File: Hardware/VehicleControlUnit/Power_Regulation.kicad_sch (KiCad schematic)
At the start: 3 parts

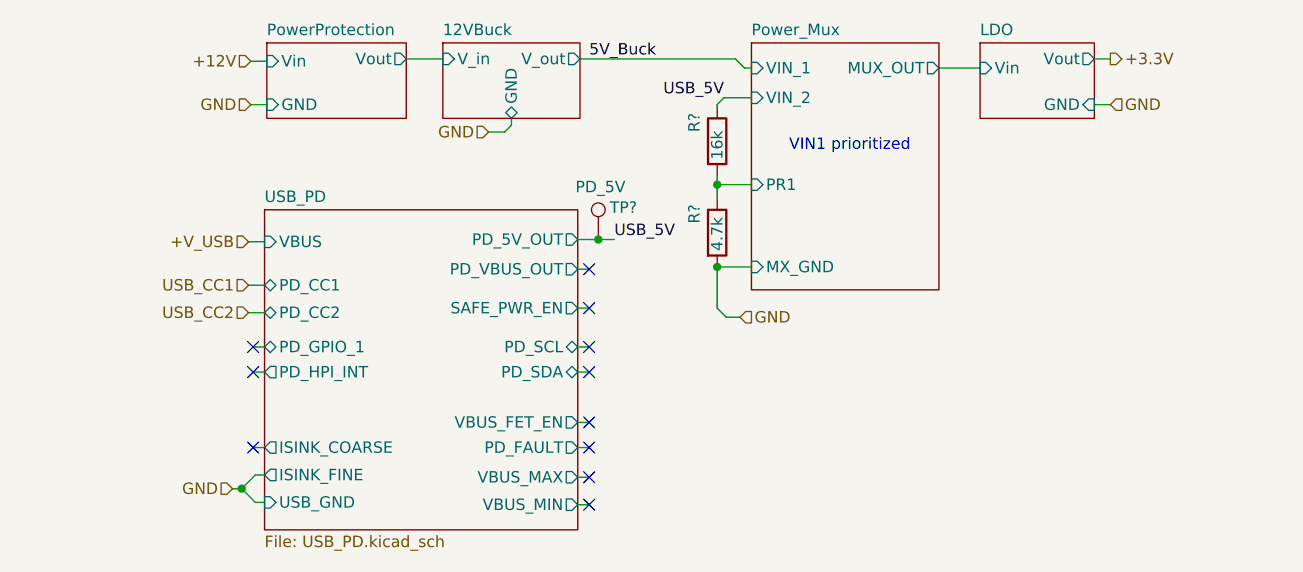
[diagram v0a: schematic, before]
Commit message: VCU more like diddle-u, mika time
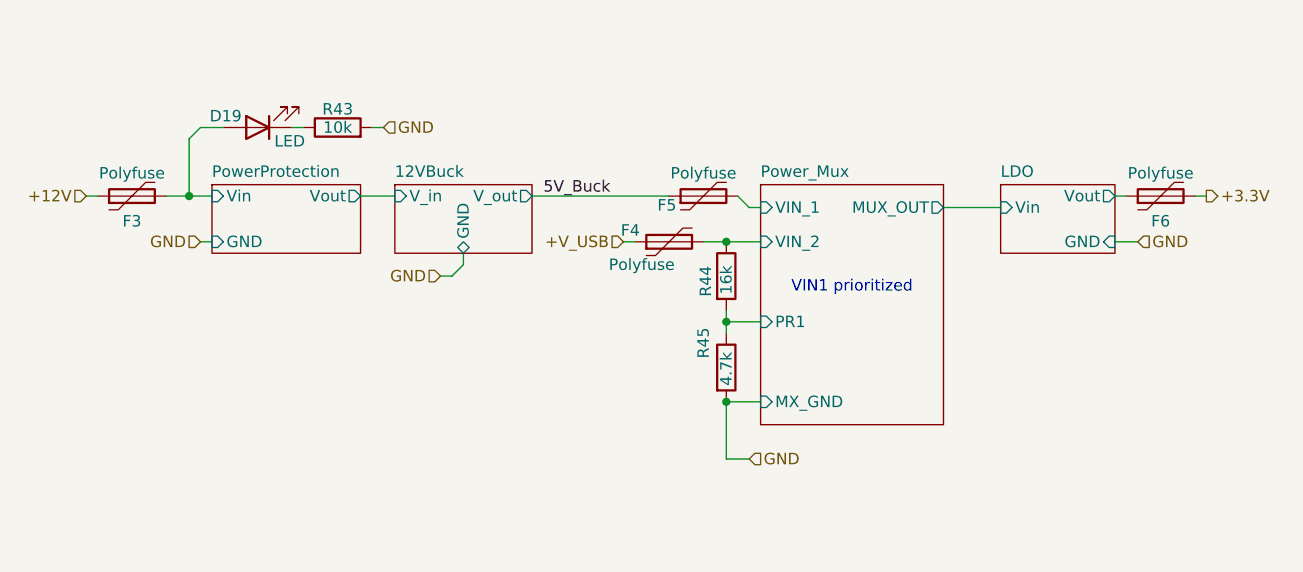
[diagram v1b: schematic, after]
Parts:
- removed TP?: PD_5V, symbol Connector:TestPoint
- added D19: LED, symbol Device:LED
- added F3, F4, F5, F6: Polyfuse, symbol Device:Polyfuse
- added R43: 10k, symbol Device:R
- gave numbers to parts that had none: 2
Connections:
- net +12V: now also F3.1
- net +3.3V: now also F6.2
- net +V_USB: now also F4.1
- net 5V_Buck: now also F5.1
- net GND: now also R43.2
- net USB_5V renamed Power_Mux/VIN_2
- net Power_Mux/VIN_2: now also F4.2
- new net: D19.1 (K), R43.1
- new net LDO/Vout: F6.1
- new net PowerProtection/Vin: D19.2 (A), F3.2
- new net Power_Mux/VIN_1: F5.2
- no-connect marks 11 -> 0
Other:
- removed sheet USB_PD
- moved on the sheet: R44, R45
